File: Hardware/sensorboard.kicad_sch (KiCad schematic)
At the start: 59 parts, among them J1 RBUS, U1 ESP32-S3, Y1 40MHz±10ppm

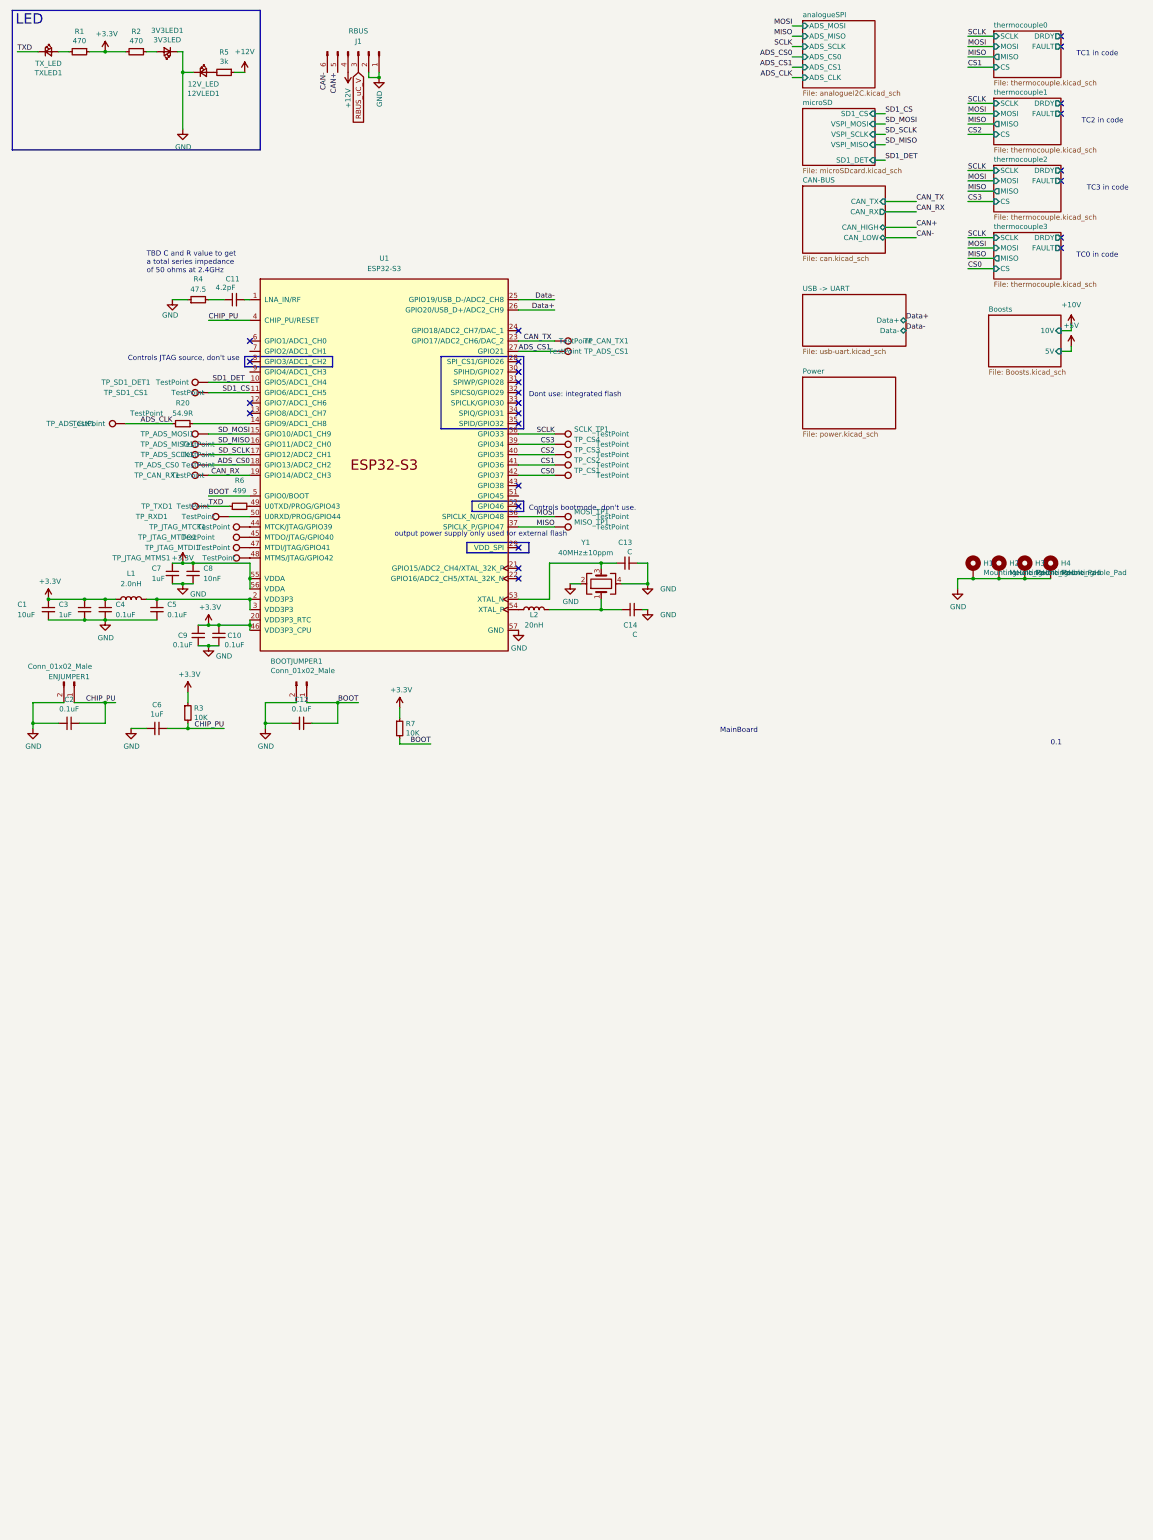
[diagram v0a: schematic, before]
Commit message: Start work
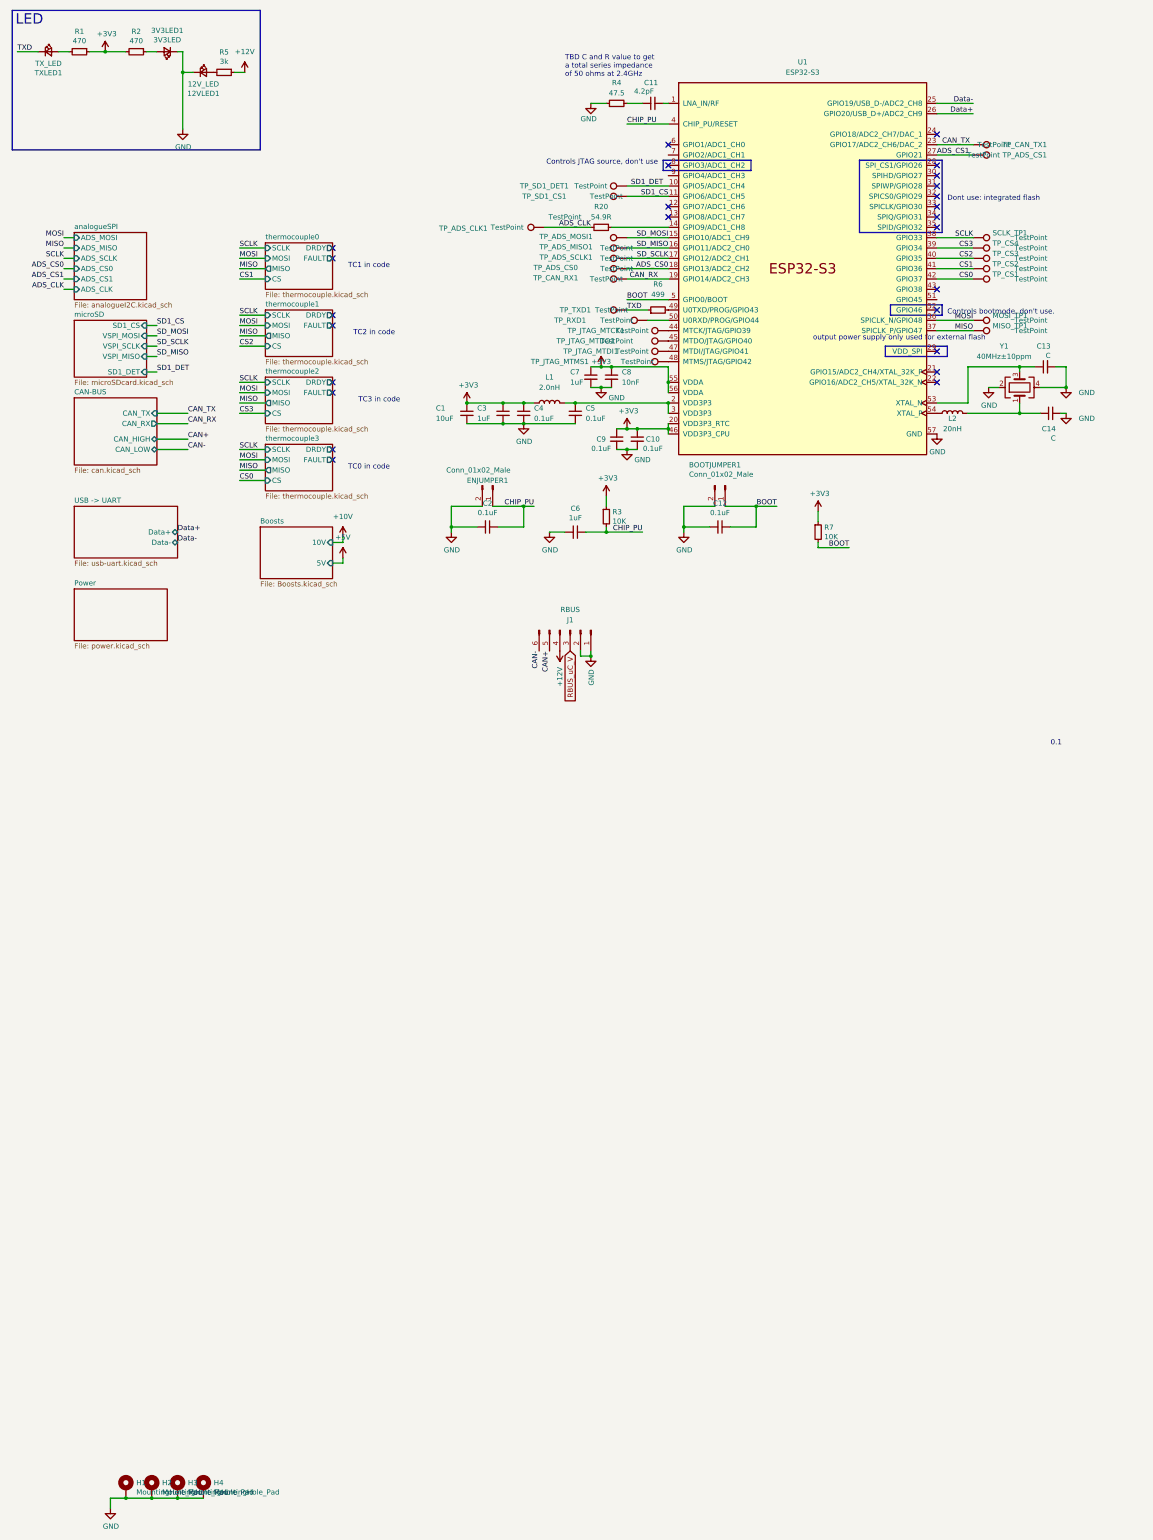
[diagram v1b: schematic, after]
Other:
- note removed: "MainBoard"
- moved on the sheet: BOOTJUMPER1, C1, C10, C11, C12, C13, C14, C2, C3, C4, C5, C6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
